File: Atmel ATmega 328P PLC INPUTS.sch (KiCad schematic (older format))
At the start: 46 parts, among them J10 Screw_Terminal_01x03, J11 Screw_Terminal_01x03, J5 Screw_Terminal_01x03, J6 Screw_Terminal_01x03, J7 Screw_Terminal_01x03, J8 Screw_Terminal_01x03, J9 Screw_Terminal_01x03, U3 PC817, U4 PC817, U5 PC817, U6 PC817, U7 PC817

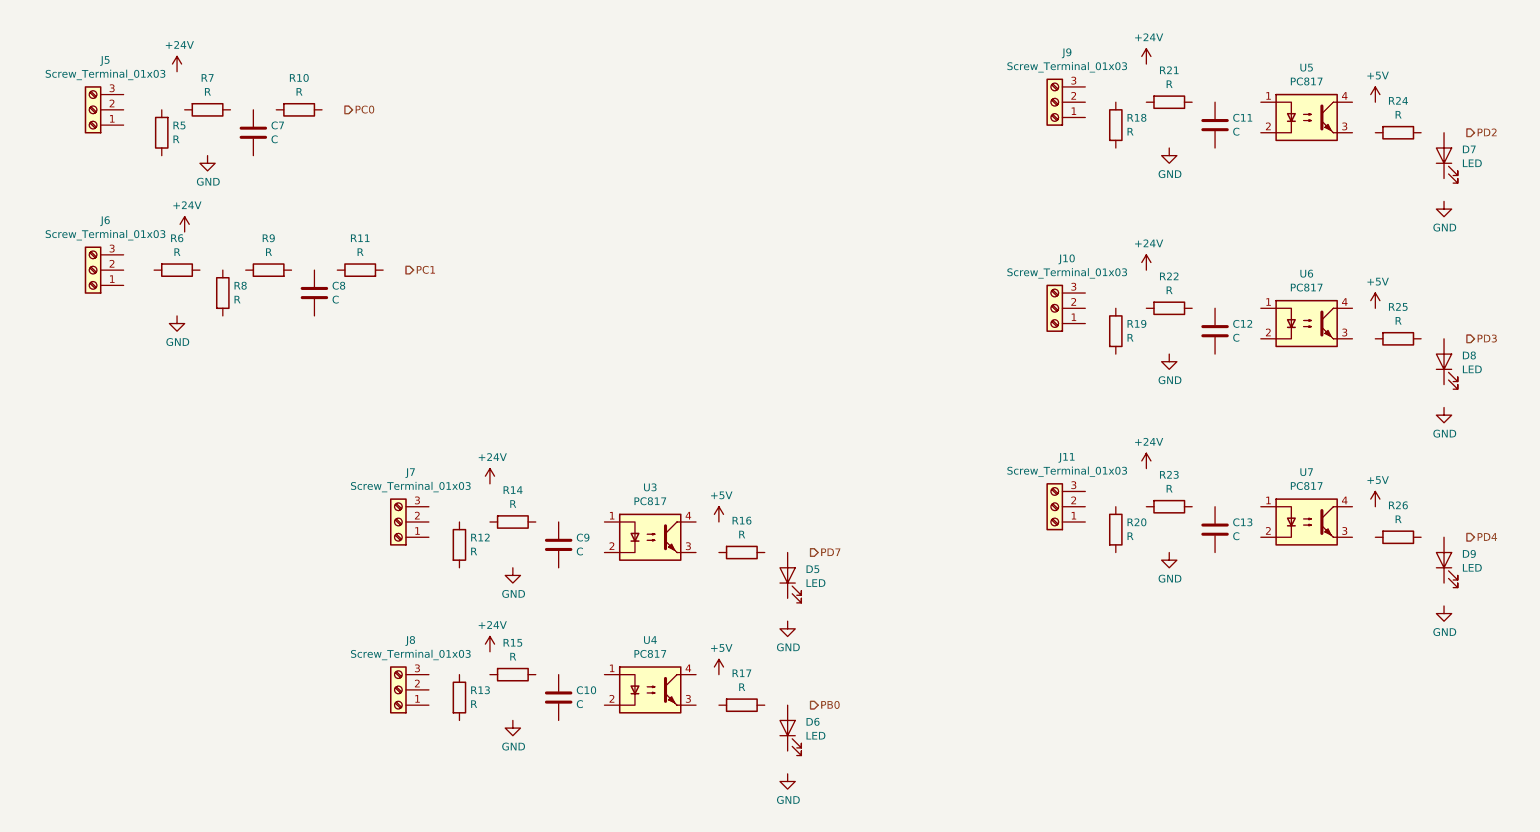
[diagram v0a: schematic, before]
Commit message: Finished schematic with all elements.
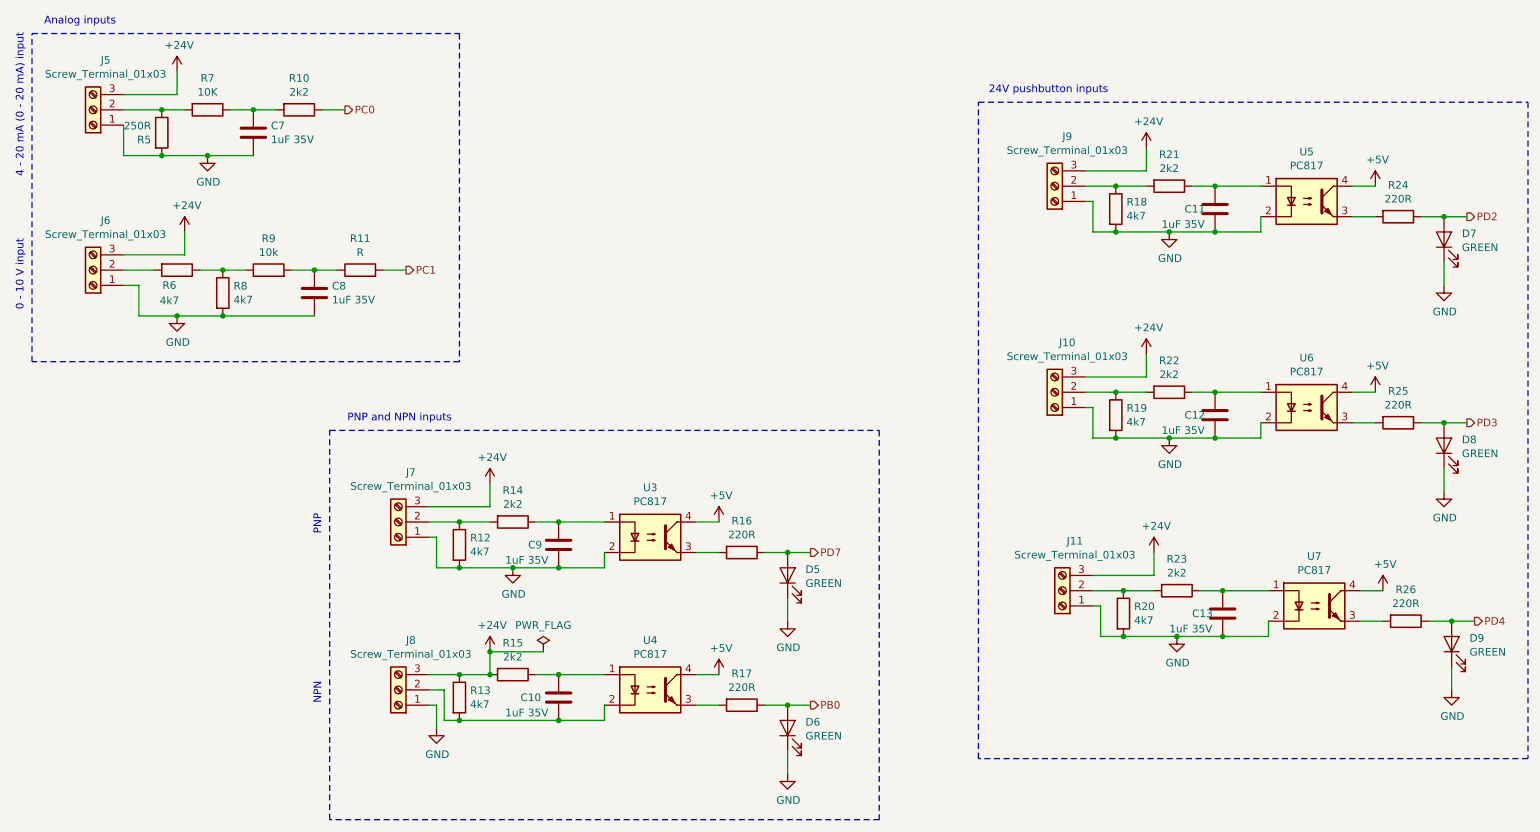
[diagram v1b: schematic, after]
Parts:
- C10, C11, C12, C13, C7, C8, C9: value C -> 1uF 35V
- D5, D6, D7, D8, D9: value LED -> GREEN
- R10, R14, R15, R21, R22, R23: value R -> 2k2
- R12, R13, R18, R19, R20, R6, R8: value R -> 4k7
- R16, R17, R24, R25, R26: value R -> 220R
- R5: value R -> 250R
- R7: value R -> 10K
- R9: value R -> 10k
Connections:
- net +24V: now also J10.3 (Pin_3), J11.3 (Pin_3), J5.3 (Pin_3), J6.3 (Pin_3), J7.3 (Pin_3), J8.3 (Pin_3), J9.3 (Pin_3), R13.1, R15.2
- net +5V: now also U3.4, U4.4, U5.4, U6.4, U7.4
- net GND: now also C11.2, C12.2, C13.2, C7.2, C8.2, C9.2, D5.1 (K), D6.1 (K), D7.1 (K), D8.1 (K), D9.1 (K), J10.1 (Pin_1), J11.1 (Pin_1), J5.1 (Pin_1), J6.1 (Pin_1), J7.1 (Pin_1), J8.1 (Pin_1), J9.1 (Pin_1), R12.2, R18.2, R19.2, R20.2, R5.2, R8.2, U3.2, U5.2, U6.2, U7.2
- net PB0: now also D6.2 (A), R17.1
- net PC0: now also R10.1
- net PC1: now also R11.2
- net PD2: now also D7.2 (A), R24.1
- net PD3: now also D8.2 (A), R25.1
- net PD4: now also D9.2 (A), R26.1
- net PD7: now also D5.2 (A), R16.1
- net at R8.1: now also R6.1, R9.1
- net at R9.2: now also C8.1, R11.1
- net at R10.2: now also C7.1, R7.1
- net at C10.1: now also R15.1, U4.1
- net at C10.2: now also J8.2 (Pin_2), R13.2, U4.2
- net at U4.3: now also R17.2
- net at R16.2: now also U3.3
- net at U3.1: now also C9.1, R14.1
- net at R24.2: now also U5.3
- net at U5.1: now also C11.1, R21.1
- net at J9.2 (Pin_2): now also R18.1, R21.2
- net at J7.2 (Pin_2): now also R12.1, R14.2
- net at R7.2: now also J5.2 (Pin_2), R5.1
- net at R6.2: now also J6.2 (Pin_2)
- net at R25.2: now also U6.3
- net at U6.1: now also C12.1, R22.1
- net at J10.2 (Pin_2): now also R19.1, R22.2
- net at R26.2: now also U7.3
- net at U7.1: now also C13.1, R23.1
- net at J11.2 (Pin_2): now also R20.1, R23.2
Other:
- note added: "0 - 10 V input"
- note added: "24V pushbutton inputs"
- note added: "4 - 20 mA (0 - 20 mA) input\n"
- note added: "Analog inputs"
- note added: "NPN\n"
- note added: "PNP"
- note added: "PNP and NPN inputs"
